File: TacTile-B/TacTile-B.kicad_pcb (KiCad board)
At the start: 2 copper layers, 59.9 x 59.9 mm, 97 parts, among them J1 Conn_01x02, J10 Conn_01x02, J11 Conn_01x02, J12 Conn_01x02, J13 Conn_01x02, J14 Conn_01x02, J15 Conn_01x02, J16 Conn_01x02, J17 Conn_01x02, J2 Conn_01x02, J3 Conn_01x02, J4 Conn_01x02, J5 Conn_01x02, J6 Conn_01x02, J7 Conn_01x02, J8 Conn_01x02, J9 Conn_01x02, U1 MCP14A0304xMNY, U10 MCP14A0304xMNY, U11 MCP14A0304xMNY, U12 MCP14A0304xMNY, U13 MCP14A0304xMNY, U14 MCP14A0304xMNY, U15 MCP14A0304xMNY, U16 MCP14A0304xMNY, U2 MCP14A0304xMNY, U3 MCP14A0304xMNY, U4 MCP14A0304xMNY, U5 MCP14A0304xMNY, U6 MCP14A0304xMNY, U7 MCP14A0304xMNY, U8 MCP14A0304xMNY, U9 MCP14A0304xMNY

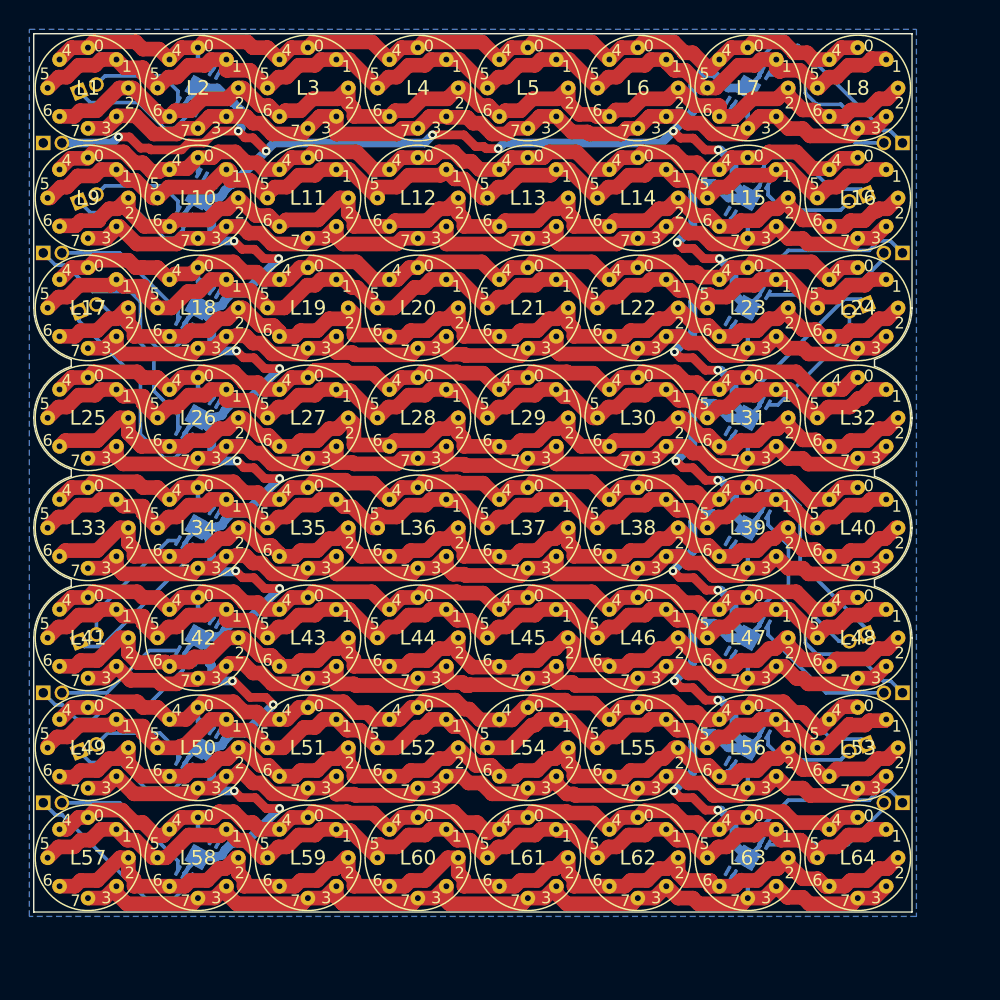
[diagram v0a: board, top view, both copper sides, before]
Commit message: Began layout and routing of board C
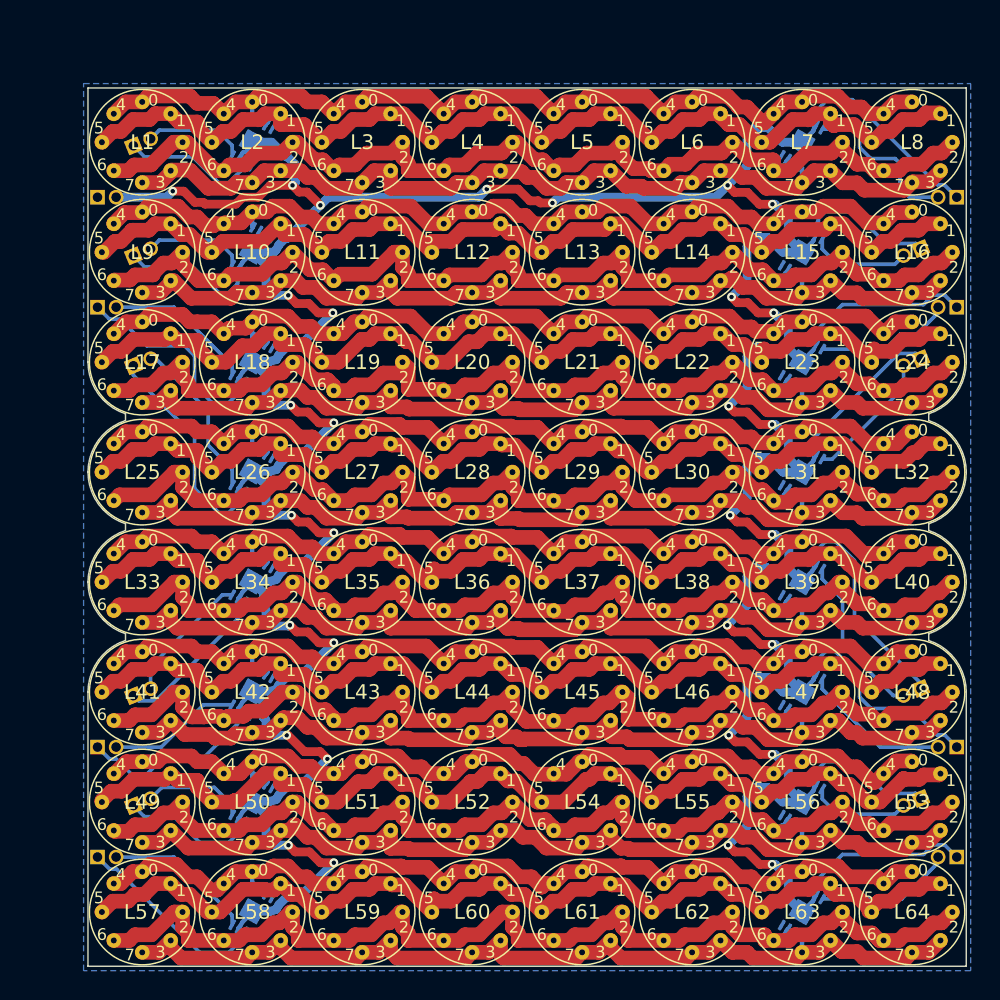
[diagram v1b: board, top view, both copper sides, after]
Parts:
- moved J10 5.23 mm to (81.8, 66.0)
- moved J12 5.23 mm to (84.2, 70.0)
- moved J14 5.23 mm to (81.8, 73.5)
- moved J16 5.23 mm to (84.2, 77.5)
- moved J2 5.23 mm to (84.2, 32.5)
- moved J6 5.23 mm to (84.2, 40.0)
- moved L10 5.23 mm to (36.2, 36.2)
- moved L11 5.23 mm to (43.7, 36.2)
- moved L12 5.23 mm to (51.2, 36.2)
- moved L13 5.23 mm to (58.7, 36.2)
- moved L14 5.23 mm to (66.2, 36.2)
- moved L15 5.23 mm to (73.7, 36.2)
- moved L16 5.23 mm to (81.2, 36.2)
- moved L18 5.23 mm to (36.2, 43.7)
- moved L19 5.23 mm to (43.7, 43.7)
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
